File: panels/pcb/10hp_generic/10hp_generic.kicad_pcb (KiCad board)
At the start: 2 copper layers, 50 x 106.8 mm, 88 parts, among them J1 CAN_PWR, J2 SWD, SW1 SW_Push, SW10 SW_Push, SW11 SW_Push, SW12 SW_Push, SW13 SW_Push, SW14 SW_Push, SW15 SW_Push, SW16 SW_Push, SW2 SW_Push, SW3 SW_Push, SW4 SW_Push, SW5 SW_Push, SW6 SW_Push, SW7 SW_Push, SW8 SW_Push, SW9 SW_Push, U1 TJA1051T-3, U2 AMS1117-3.3, U3 STM32F103C8Tx, Y1 8MHz

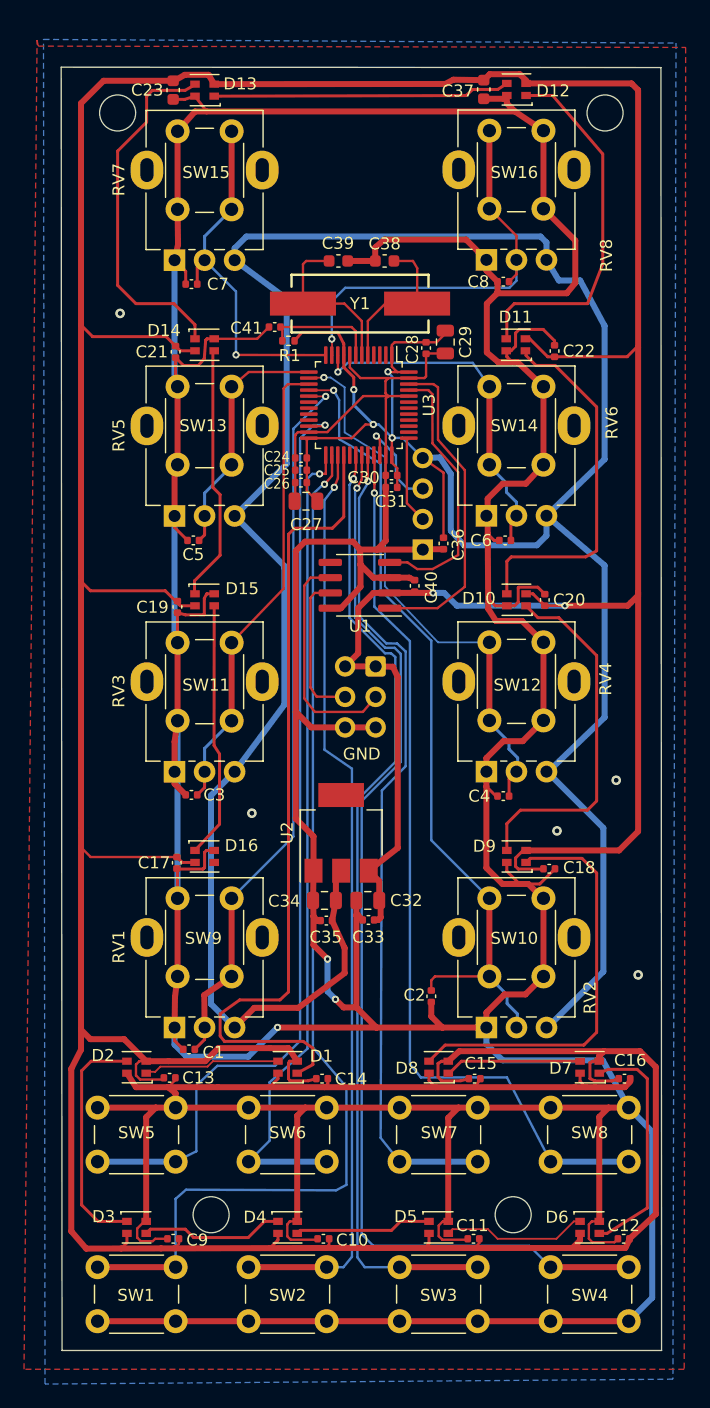
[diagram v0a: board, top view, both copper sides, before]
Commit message: Rev 3 boards complete - probably
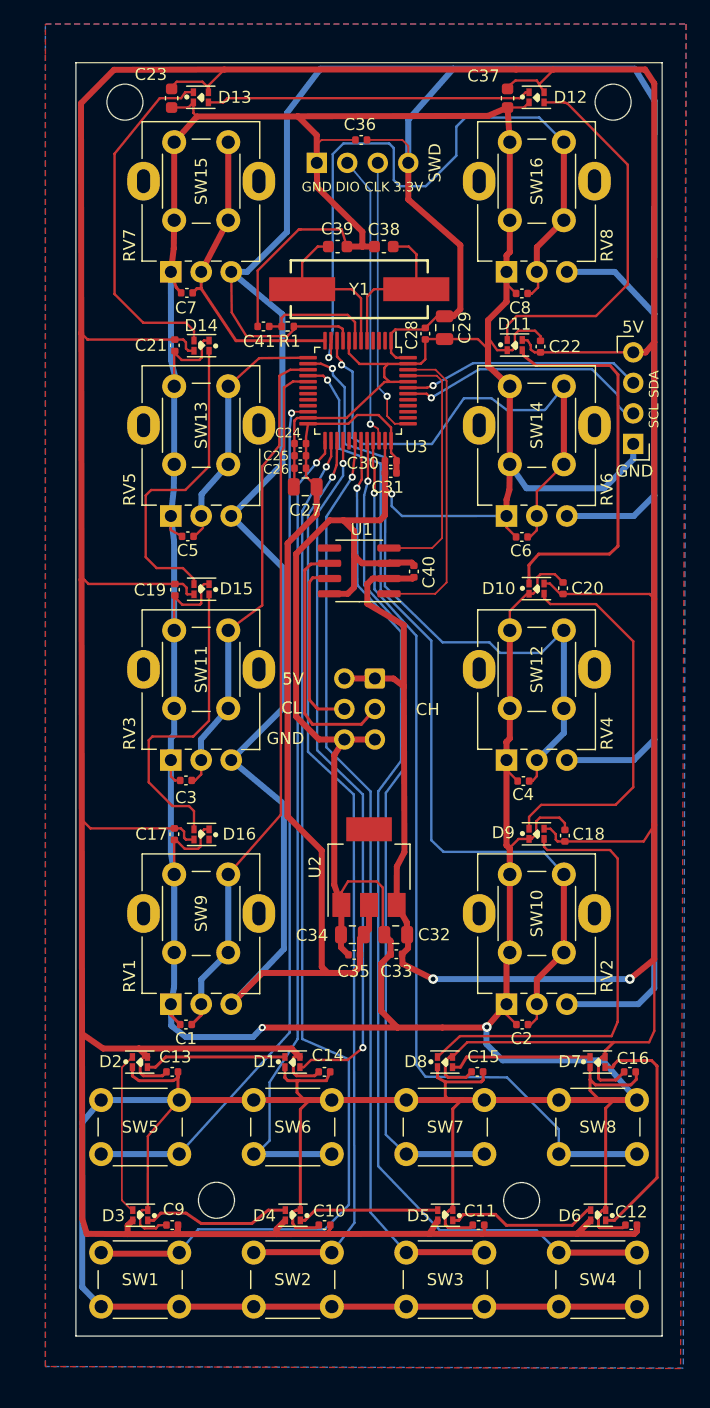
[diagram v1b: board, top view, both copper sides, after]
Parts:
- added J3: I2C, Connector_PinHeader_2.54mm:PinHeader_1x04_P2.54mm_Vertical, F.Cu at (98.3, 75.4)
- C38, C39: value 20pF -> 22pF
- D1, D10, D11, D12, D13, D14, D15, D16, D2, D3, D4, D5, D6, D7, D8, D9: footprint WS2812:XL-2121RGBC-WS2812B -> riban:LED_XL-1615RGBC-WS2812B
- SW1, SW10, SW11, SW12, SW13, SW14, SW15, SW16, SW2, SW3, SW4, SW5, SW6, SW7, SW8, SW9: footprint Button_Switch_THT:SW_PUSH_6mm_H4.3mm -> riban:SW_PUSH_6mm_H4.3mm
- moved C36 34.3 mm to (75.6, 50.1), turned to 180 degrees
- moved J2 33.4 mm to (71.9, 52.0), turned to -90 degrees
- moved RV2 10.4 mm to (90.3, 114.5)
- moved RV1 9.75 mm to (62.3, 114.5)
- moved RV4 9.49 mm to (90.3, 94.2)
- moved RV3 8.81 mm to (62.3, 94.2)
- moved RV6 8.62 mm to (90.3, 73.9)
- moved C2 7.93 mm to (89.1, 123.8), turned to 0 degrees
- moved RV5 7.87 mm to (62.3, 73.9)
- moved RV8 7.78 mm to (90.3, 53.6)
- moved RV7 6.94 mm to (62.3, 53.6)
- moved SW9 5.60 mm to (62.3, 114.5)
- moved SW11 4.71 mm to (62.3, 94.2)
- moved SW1 4.55 mm to (57.2, 145.0)
- moved SW2 4.47 mm to (70.0, 145.0)
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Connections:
- D1 pad 1: GND -> Net-(D1-Pad1)
- D1 pad 2: WS2812 -> +5V
- D1 pad 3: +5V -> GND
- D1 pad 4: Net-(D1-Pad4) -> WS2812
- D10 pad 1: GND -> Net-(D10-Pad1)
- D10 pad 2: Net-(D10-Pad2) -> +5V
- D10 pad 3: +5V -> GND
- D11 pad 1: GND -> Net-(D11-Pad1)
- D11 pad 2: Net-(D10-Pad4) -> +5V
- D11 pad 3: +5V -> GND
- D11 pad 4: Net-(D11-Pad4) -> Net-(D10-Pad1)
- D12 pad 1: GND -> Net-(D12-Pad1)
- D12 pad 2: Net-(D11-Pad4) -> +5V
- D12 pad 3: +5V -> GND
- D12 pad 4: Net-(D12-Pad4) -> Net-(D11-Pad1)
- D13 pad 1: GND -> Net-(D13-Pad1)
- D13 pad 2: Net-(D12-Pad4) -> +5V
- D13 pad 3: +5V -> GND
- D13 pad 4: Net-(D13-Pad4) -> Net-(D12-Pad1)
- D14 pad 1: GND -> Net-(D14-Pad1)
- D14 pad 2: Net-(D13-Pad4) -> +5V
- D14 pad 3: +5V -> GND
- D14 pad 4: Net-(D14-Pad4) -> Net-(D13-Pad1)
- D15 pad 1: GND -> Net-(D15-Pad1)
- D15 pad 2: Net-(D14-Pad4) -> +5V
- D15 pad 3: +5V -> GND
- D15 pad 4: Net-(D15-Pad4) -> Net-(D14-Pad1)
- D16 pad 1: GND -> unconnected-(D16-Pad1)
- D16 pad 2: Net-(D15-Pad4) -> +5V
- D16 pad 3: +5V -> GND
- D16 pad 4: unconnected-(D16-Pad4) -> Net-(D15-Pad1)
- D2 pad 1: GND -> Net-(D2-Pad1)
- D2 pad 2: Net-(D1-Pad4) -> +5V
- D2 pad 3: +5V -> GND
- D2 pad 4: Net-(D2-Pad4) -> Net-(D1-Pad1)
- D3 pad 1: GND -> Net-(D3-Pad1)
- D3 pad 2: Net-(D2-Pad4) -> +5V
- D3 pad 3: +5V -> GND
- D3 pad 4: Net-(D3-Pad4) -> Net-(D2-Pad1)
- D4 pad 1: GND -> Net-(D4-Pad1)
- D4 pad 2: Net-(D3-Pad4) -> +5V
- D4 pad 3: +5V -> GND
- D4 pad 4: Net-(D4-Pad4) -> Net-(D3-Pad1)
- D5 pad 1: GND -> Net-(D5-Pad1)
- D5 pad 2: Net-(D4-Pad4) -> +5V
- D5 pad 3: +5V -> GND
- D5 pad 4: Net-(D5-Pad4) -> Net-(D4-Pad1)
- D6 pad 1: GND -> Net-(D6-Pad1)
- D6 pad 2: Net-(D5-Pad4) -> +5V
- D6 pad 3: +5V -> GND
- D6 pad 4: Net-(D6-Pad4) -> Net-(D5-Pad1)
- D7 pad 1: GND -> Net-(D7-Pad1)
- D7 pad 2: Net-(D6-Pad4) -> +5V
- D7 pad 3: +5V -> GND
- D7 pad 4: Net-(D7-Pad4) -> Net-(D6-Pad1)
- D8 pad 1: GND -> Net-(D8-Pad1)
- D8 pad 2: Net-(D7-Pad4) -> +5V
- D8 pad 3: +5V -> GND
- D8 pad 4: Net-(D8-Pad4) -> Net-(D7-Pad1)
- D9 pad 1: GND -> Net-(D10-Pad4)
- D9 pad 2: Net-(D8-Pad4) -> +5V
- D9 pad 3: +5V -> GND
- D9 pad 4: Net-(D10-Pad2) -> Net-(D8-Pad1)
- J2 pad 2: SWCLK -> SWDIO
- J2 pad 3: SWDIO -> SWCLK
- U3 pad 42: SDA -> SCL
- U3 pad 43: SCL -> SDA
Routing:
- net VDD: track 272.5 -> 360.0 mm, vias 4 -> 0
- net Net-(D8-Pad1): track 0.00 -> 37.3 mm
- net Net-(D8-Pad4): track 34.7 -> 0.00 mm
- net Net-(D10-Pad1): track 0.00 -> 32.9 mm
- net Net-(D11-Pad1): track 0.00 -> 31.7 mm
- net Net-(D11-Pad4): track 30.6 -> 0.00 mm
- net Net-(D10-Pad2): track 30.2 -> 0.00 mm
- net Net-(D13-Pad4): track 30.2 -> 0.00 mm
- net Net-(D13-Pad1): track 0.00 -> 29.4 mm
- net GND: track 686.9 -> 657.7 mm, vias 8 -> 3
- net Net-(D12-Pad1): track 0.00 -> 27.0 mm
- net Net-(D14-Pad1): track 0.00 -> 26.2 mm
- net Net-(D15-Pad1): track 0.00 -> 26.0 mm
- net Net-(D12-Pad4): track 24.7 -> 0.00 mm
- net +5V: track 449.8 -> 474.2 mm
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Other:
- board size 50 x 106.8 mm -> 48.8 x 106 mm
- rule pad_to_mask_clearance: 0 -> 0.05
- board text added: "3.3V"
- board text added: "CLK"
- board text added: "DIO"
- board text added: "SCL"
- board text added: "SDA"
- board text removed: "+3V"
- board text removed: "SWCLK"
- board text removed: "SWDIO"
